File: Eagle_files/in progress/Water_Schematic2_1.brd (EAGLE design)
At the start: 36.8 x 52.6 mm, 12 parts

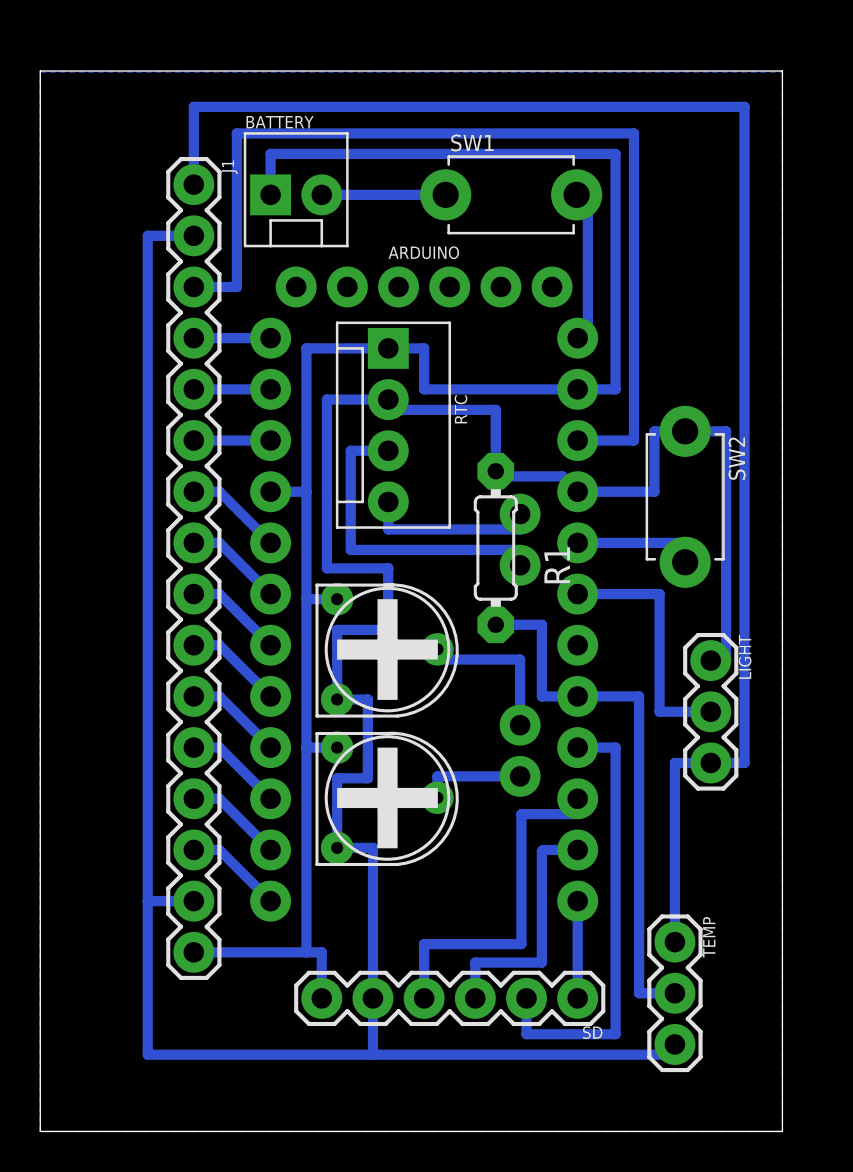
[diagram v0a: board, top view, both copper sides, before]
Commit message: almost there brd
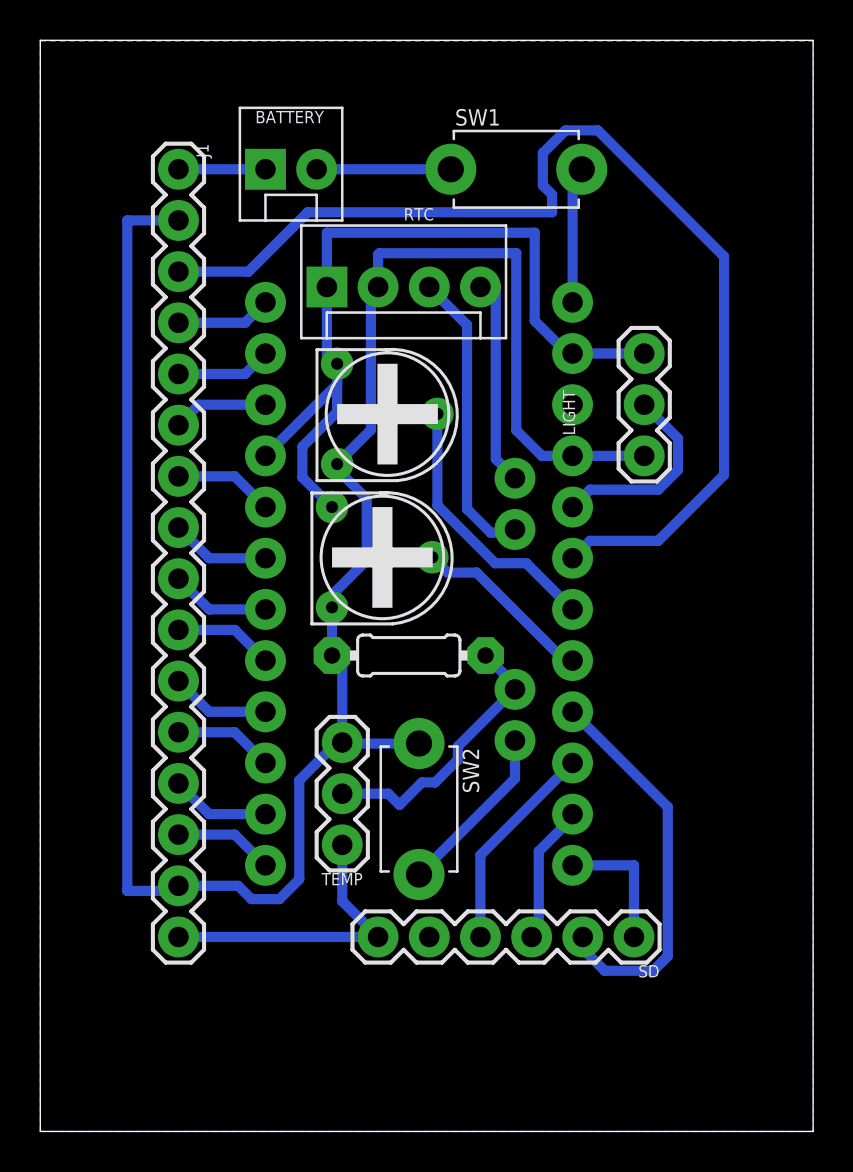
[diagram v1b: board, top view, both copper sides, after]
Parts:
- removed ARDUINO: ARDUINO_PRO_MINI, SparkFun-Boards:ARDUINO_PRO_MINI
- added B1: ARDUINO_PRO_MINI, SparkFun-Boards_mod:ARDUINO_PRO_MINI
- moved SW2 20.4 mm to (18.8, 16.0)
- moved TEMP 17.2 mm to (15.0, 14.2), turned to 90 degrees
- moved POT1 11.9 mm to (14.5, 31.0)
- moved POT2 11.7 mm to (14.7, 38.1)
- moved LIGHT 10.7 mm to (30.0, 33.5), turned to 90 degrees
- moved R1 6.86 mm to (18.3, 23.6), turned to 180 degrees
- moved RTC 4.31 mm to (14.2, 41.9), turned to 0 degrees
- moved SD 4.13 mm to (29.5, 9.65)
- moved SW1 1.30 mm to (23.6, 47.8)
- moved BATTERY 1.30 mm to (11.2, 47.8)
- moved J1 1.08 mm to (6.86, 47.8)
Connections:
- removed net A4: ARDUINO.19, LIGHT.2
- removed net VEE: ARDUINO.22, J1.3
- new net A1: B1.18, POT2.OUT
- new net A2: B1.19, J1.3
- new net RST: B1.22
- net A0: now also B1.17, POT1.OUT; no longer ARDUINO.17, R1.1, TEMP.2
- net A3: now also B1.20, LIGHT.2; no longer ARDUINO.20, SW2.P$2
- net A6: now also B1.A6, SW2.P$2; no longer ARDUINO.A6, POT1.OUT
- net A7: now also B1.A7, R1.1, TEMP.2; no longer ARDUINO.A7, POT2.OUT
- net E: now also B1.3; no longer ARDUINO.3
- net GND: now also B1.23, B1.4; no longer ARDUINO.23, ARDUINO.4
- net L1: now also B1.5; no longer ARDUINO.5
- net L2: now also B1.6; no longer ARDUINO.6
- net L3: now also B1.7; no longer ARDUINO.7
- net L4: now also B1.8; no longer ARDUINO.8
- net L5: now also B1.9; no longer ARDUINO.9
- net L6: now also B1.10; no longer ARDUINO.10
- net L7: now also B1.11; no longer ARDUINO.11
- net L8: now also B1.12; no longer ARDUINO.12
- net MISO: now also B1.15; no longer ARDUINO.15
- net MOSI: now also B1.14; no longer ARDUINO.14
- net RS: now also B1.1; no longer ARDUINO.1
- net RW: now also B1.2; no longer ARDUINO.2
- net SC: now also B1.13; no longer ARDUINO.13
- net SCK: now also B1.16; no longer ARDUINO.16
- net SCL: now also B1.A5; no longer ARDUINO.A5
- net SDA: now also B1.A4; no longer ARDUINO.A4
- net VCC: now also B1.21; no longer ARDUINO.21
- net VIN: now also B1.24; no longer ARDUINO.24
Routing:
- net GND: track 168.5 -> 61.8 mm
- net A2: track 0.00 -> 55.0 mm
- net VCC: track 153.7 -> 106.0 mm
- net VEE: track 47.5 -> 0.00 mm
- net A0: track 27.5 -> 9.08 mm
- net A1: track 0.00 -> 13.4 mm
- net A4: track 12.4 -> 0.00 mm
- net MISO: track 17.4 -> 10.5 mm
- net A7: track 7.87 -> 13.8 mm
- net MOSI: track 12.4 -> 6.94 mm
- net A3: track 6.30 -> 9.93 mm
- net A6: track 5.16 -> 8.62 mm
- net SCK: track 22.3 -> 19.6 mm
- net SCL: track 8.67 -> 10.6 mm
- net SC: track 4.83 -> 6.60 mm
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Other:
- board size 36.8 x 52.6 mm -> 38.4 x 54.2 mm

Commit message: almost there!!!!!!
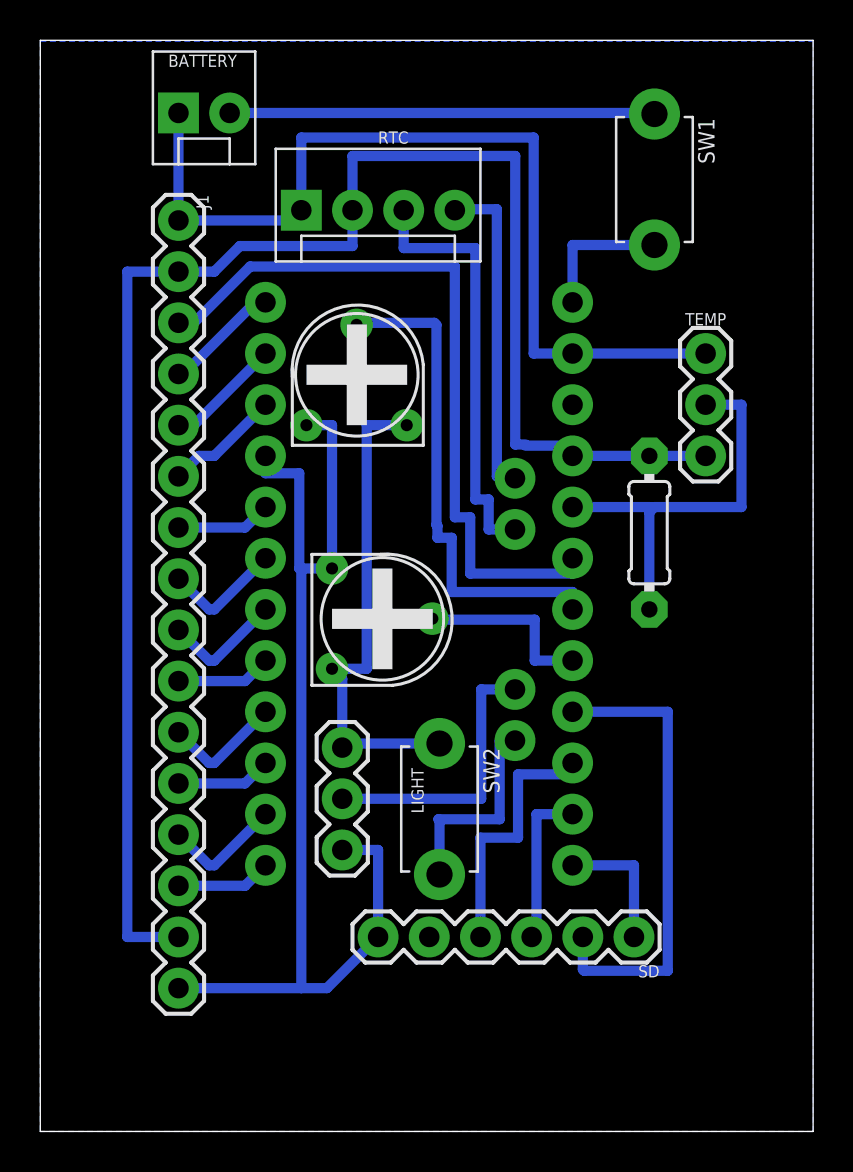
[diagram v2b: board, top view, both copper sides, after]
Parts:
- moved TEMP 30.3 mm to (33.0, 38.6), turned to 270 degrees
- moved LIGHT 20.8 mm to (15.0, 19.1), turned to 270 degrees
- moved R1 13.4 mm to (30.2, 29.7), turned to 90 degrees
- moved SW1 6.88 mm to (30.5, 47.2), turned to 270 degrees
- moved BATTERY 5.14 mm to (6.86, 50.5)
- moved RTC 4.02 mm to (13.0, 45.7)
- moved POT2 3.41 mm to (13.2, 35.1), turned to 0 degrees
- moved POT1 3.05 mm to (14.5, 27.9)
- moved J1 2.54 mm to (6.86, 45.2)
- moved SW2 1.02 mm to (19.8, 16.0)
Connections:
- net A3: now also R1.1, TEMP.2; no longer LIGHT.2
- net A7: now also LIGHT.2; no longer R1.1, TEMP.2
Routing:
- net GND: track 61.8 -> 101.5 mm
- net A2: track 55.0 -> 36.7 mm
- net BAT: track 6.66 -> 21.1 mm
- net A1: track 13.4 -> 24.9 mm
- net A3: track 9.93 -> 20.4 mm
- net SDA: track 14.7 -> 21.4 mm
- net SCL: track 10.6 -> 16.3 mm
- net SCK: track 19.6 -> 23.4 mm
- net VCC: track 106.0 -> 109.6 mm
- net MISO: track 10.5 -> 13.2 mm
- net A6: track 8.62 -> 10.5 mm
- net MOSI: track 6.94 -> 8.13 mm
- net L3: track 4.95 -> 6.00 mm
- net RW: track 4.74 -> 5.79 mm
- net RS: track 4.74 -> 5.79 mm
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
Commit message: got the latest schematic working
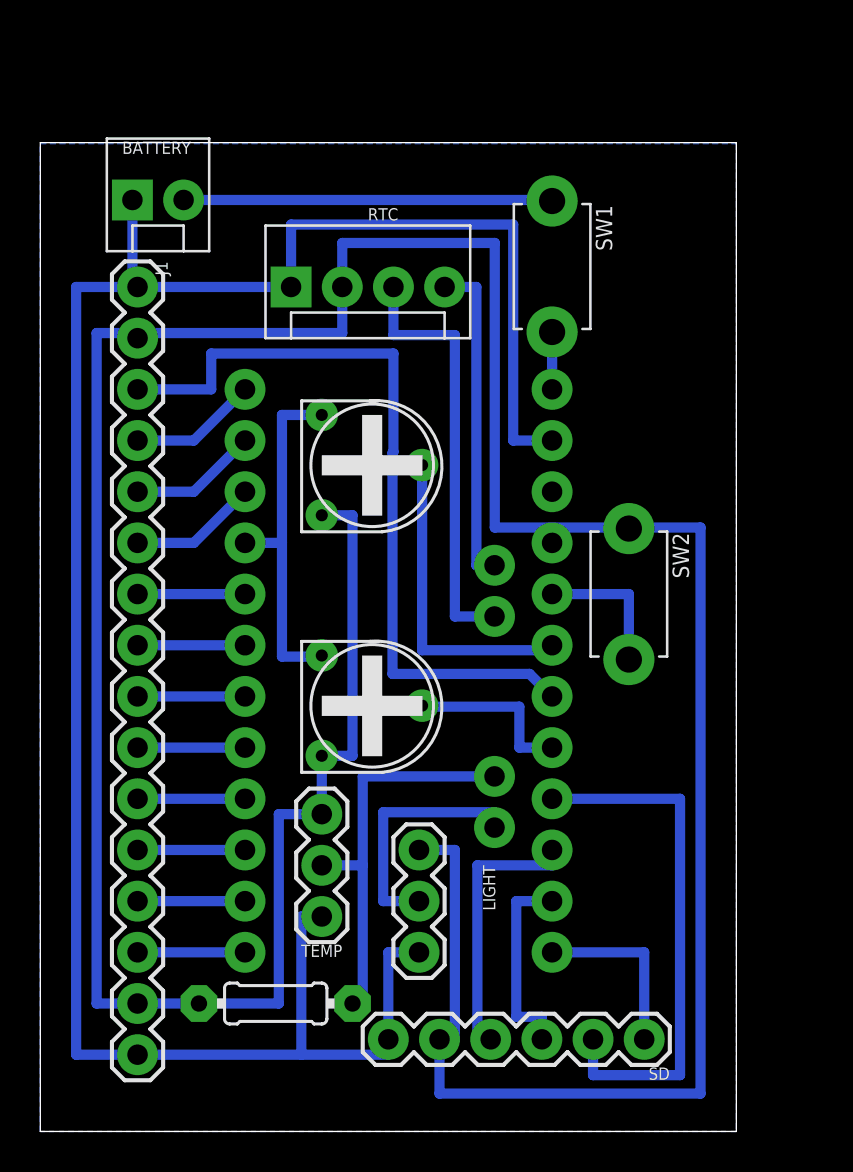
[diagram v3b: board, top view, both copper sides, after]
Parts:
- moved TEMP 33.8 mm to (14.0, 10.7), turned to 90 degrees
- moved R1 29.8 mm to (11.7, 6.35), turned to 180 degrees
- moved SW2 14.2 mm to (29.2, 26.7)
- moved SW1 6.67 mm to (25.4, 42.9)
- moved LIGHT 6.35 mm to (18.8, 14.0)
- moved SD 5.11 mm to (30.0, 4.57)
- moved BATTERY 4.89 mm to (4.57, 46.2)
- moved B1 4.44 mm to (17.8, 24.1)
- moved POT1 4.35 mm to (14.0, 23.6)
- moved J1 3.88 mm to (4.83, 41.9)
- moved RTC 3.84 mm to (12.4, 41.9)
- moved POT2 0.92 mm to (14.0, 35.6), turned to 270 degrees
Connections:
- net A1: now also J1.3; no longer POT2.OUT
- net A2: now also POT2.OUT; no longer J1.3
- net A3: now also SW2.P$2; no longer R1.1, TEMP.2
- net A6: now also LIGHT.2; no longer SW2.P$2
- net A7: now also R1.1, TEMP.2; no longer LIGHT.2
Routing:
- net VCC: track 109.6 -> 177.1 mm
- net GND: track 101.5 -> 127.7 mm
- net A2: track 36.7 -> 15.9 mm
- net A1: track 24.9 -> 38.8 mm
- net A3: track 20.4 -> 7.06 mm
- net A7: track 14.0 -> 20.4 mm
- net VIN: track 6.91 -> 2.85 mm
- net BAT: track 21.1 -> 18.3 mm
- net SCK: track 23.4 -> 26.2 mm
- net SC: track 6.60 -> 8.89 mm
- net A6: track 10.5 -> 12.5 mm
- net MOSI: track 8.13 -> 9.91 mm
- net A0: track 9.43 -> 8.53 mm
- net L3: track 6.00 -> 5.33 mm
- net L5: track 6.00 -> 5.33 mm
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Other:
- board size 38.4 x 54.2 mm -> 34.5 x 49.1 mm

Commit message: attempt 2 lcd
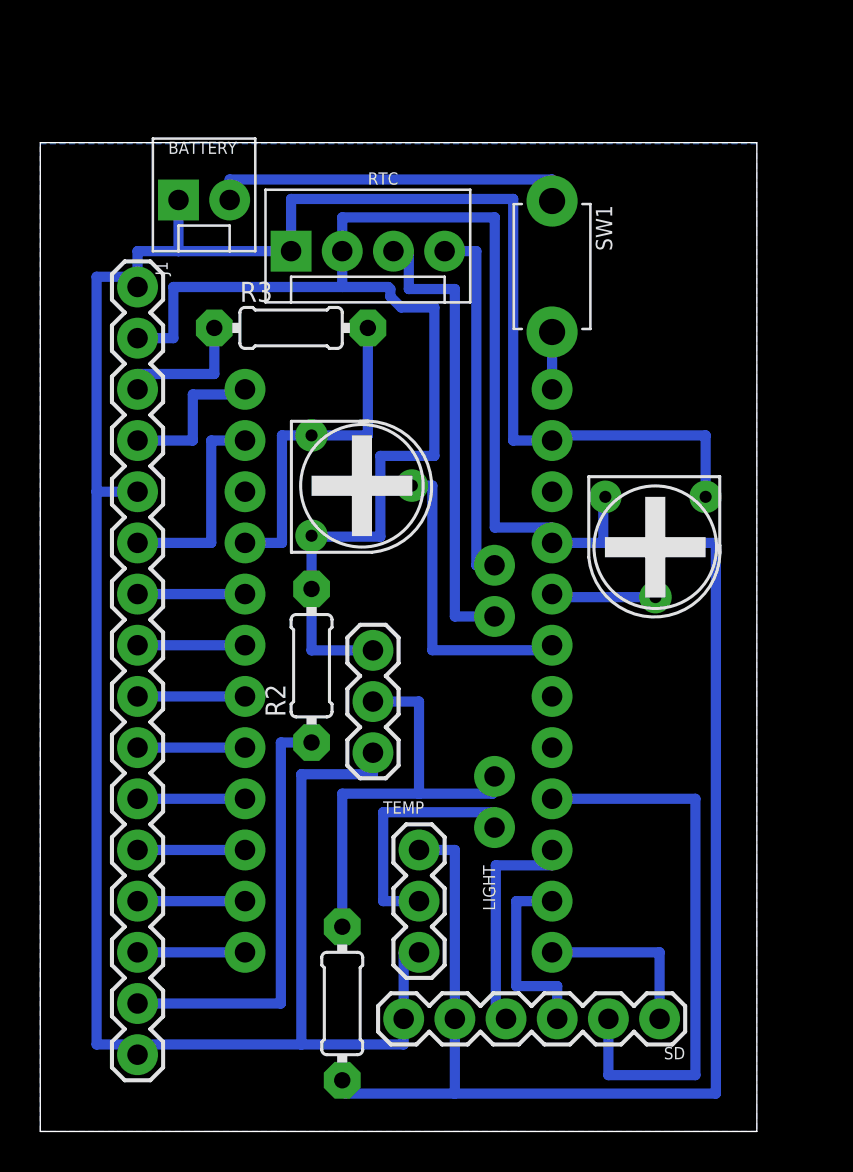
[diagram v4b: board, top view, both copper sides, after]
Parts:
- removed SW2: (no value), adafruit:TACT_PANA-EVQ
- added R2: 220, rcl:0204/7
- added R3: 1.4k, rcl:0204/7
- moved POT1 20.6 mm to (33.0, 31.5), turned to 180 degrees
- moved TEMP 8.52 mm to (16.5, 18.8)
- moved R1 3.30 mm to (15.0, 6.35), turned to 270 degrees
- moved BATTERY 2.29 mm to (6.86, 46.2)
- moved RTC 1.78 mm to (12.4, 43.7)
- moved SD 1.27 mm to (30.7, 5.59)
- moved POT2 1.14 mm to (13.5, 34.5)
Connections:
- net L1 renamed D0
- net L2 renamed D1
- net L3 renamed D2
- net L4 renamed D3
- net L5 renamed D4
- net L6 renamed D5
- net L7 renamed D6
- net L8 renamed D7
- removed net A0: B1.17, POT1.OUT
- removed net A1: B1.18, J1.3
- removed net RST: B1.22
- removed net RW: B1.2, J1.5
- new net BL: J1.15, R2.1
- new net V0: J1.3, R3.1
- net A3: now also POT1.OUT; no longer SW2.P$2
- net E: now also B1.2; no longer B1.3
- net GND: now also J1.5, R3.2
- net VCC: now also R2.2; no longer J1.15, SW2.P$1
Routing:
- net A1: track 38.8 -> 0.00 mm
- net VCC: track 177.1 -> 145.0 mm
- net BL: track 0.00 -> 21.6 mm
- net GND: track 127.7 -> 149.1 mm
- net A0: track 8.53 -> 0.00 mm
- net V0: track 0.00 -> 6.86 mm
- net RW: track 6.39 -> 0.00 mm
- net E: track 6.39 -> 10.4 mm
- net MISO: track 13.8 -> 11.7 mm
- net A3: track 7.06 -> 5.19 mm
- net SDA: track 21.4 -> 23.1 mm
- net SCL: track 16.3 -> 18.1 mm
- net SCK: track 26.2 -> 27.9 mm
- net A7: track 20.4 -> 21.9 mm
- net RS: track 6.39 -> 7.87 mm
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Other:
- board size 34.5 x 49.1 mm -> 35.6 x 49.1 mm
